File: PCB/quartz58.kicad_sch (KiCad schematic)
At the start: 194 parts, among them J1 OLED_128x32, J2 OLED_128x32, J3 Conn_01x10_Socket, J4 Conn_01x10_Pin, SW1 SW_SPDT, SW2 SW_Push, SW3 SW_SPDT, SW4 SW_Push, T1 TPS65-201A-S, U1 Nice_Nano_V2, U2 Nice_Nano_V2

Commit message: updates to pcb and BOM
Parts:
- removed D100, D101, D102, D103, D104, D105, D106, D107, D108, D109, D110, D111, D112, D113, D114, D115, D116, D117, D118, D119, D120, D34, D35, D36, D37, D38, D39, D40, D41, D42, D43, D44, D45, D46, D47, D48, D49, D50, D51, D52, D53, D54, D55, D56, D57, D58, D59, D60, D61, D62, D92, D93, D94, D95, D96, D97, D98, D99: LED_SK6812MINI, Keebio-Parts.pretty-master:SK6812-MINI-E, symbol ScottoKeebs:LED_SK6812MINI
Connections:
- net L-RGB is gone; now on net L-CS: U1.1
- net L-RGBGND is gone; now on net GND: U1.4 (GND)
- net R-RGBGND is gone; now on net GND: U2.4 (GND)
- net L-CS: no longer U1.2 (0)
- net SW1: now also U1.2 (0); no longer U1.25 (1)
- net L-RAW: no longer names the net of SW1.2 (B), U1.24 (B+)
- net R-RAW: no longer names the net of SW3.2 (B), U2.24 (B+)
- net R-RGB: no longer names the net of U2.1
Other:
- note removed: "RGB"
- moved on the sheet: BT1, BT2, D1, D10, D11, D12, D13, D14, D15, D16, D17, D18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

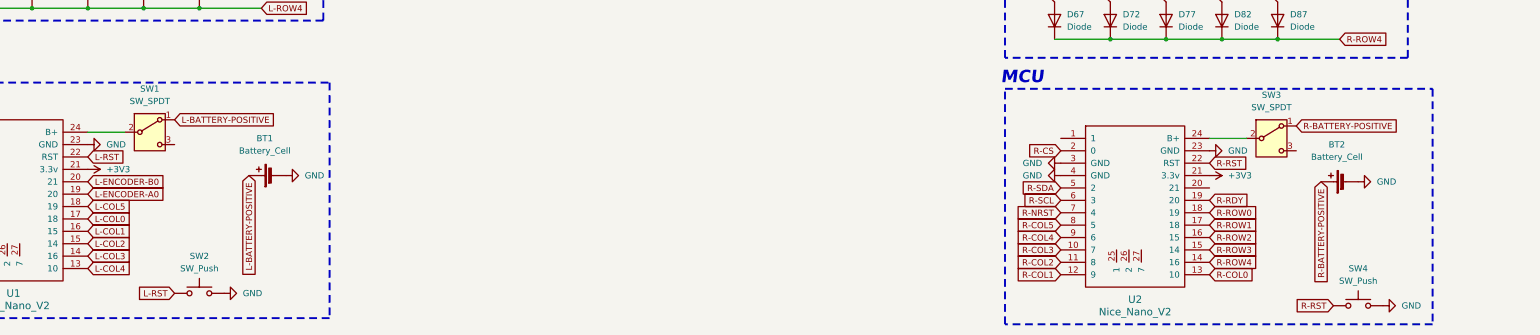
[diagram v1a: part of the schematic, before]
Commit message: borderline, caught between the tides of pain and rapture
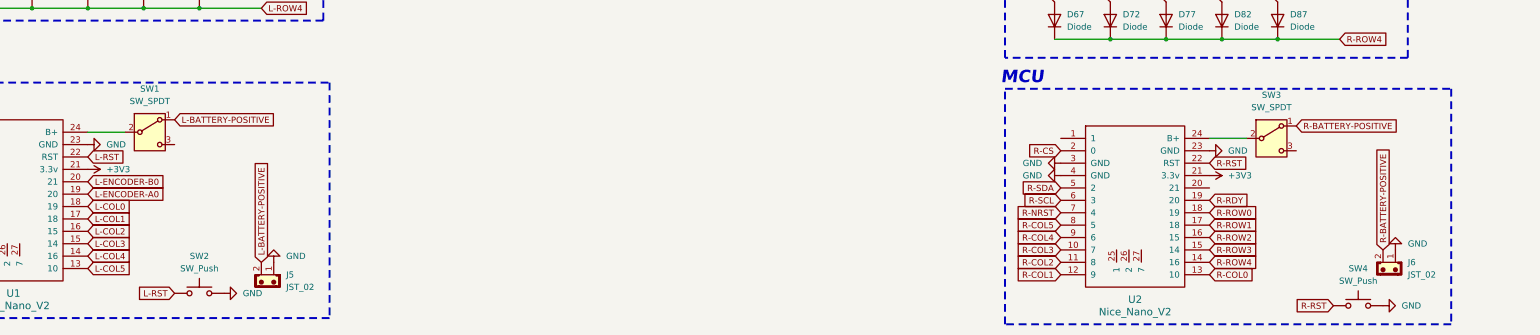
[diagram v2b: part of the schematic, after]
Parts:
- removed BT1, BT2: Battery_Cell, Connector_JST:JST_PH_S2B-PH-K_1x02_P2.00mm_Horizontal, symbol Device:Battery_Cell
- added J5, J6: JST_02, Connector_JST:JST_PH_S2B-PH-K_1x02_P2.00mm_Horizontal, symbol PCM_SL_Connectors:JST_02
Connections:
- net GND: now also J5.1, J6.1
- net L-BATTERY-POSITIVE: now also J5.2
- net L-COL0: now also U1.18 (19); no longer U1.17 (18)
- net L-COL1: now also U1.17 (18); no longer U1.16 (15)
- net L-COL2: now also U1.16 (15); no longer U1.15 (14)
- net L-COL3: now also U1.15 (14); no longer U1.14 (16)
- net L-COL4: now also U1.14 (16); no longer U1.13 (10)
- net L-COL5: now also U1.13 (10); no longer U1.18 (19)
- net R-BATTERY-POSITIVE: now also J6.2
